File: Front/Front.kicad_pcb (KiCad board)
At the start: 2 copper layers, 75 x 75 mm, 0 parts

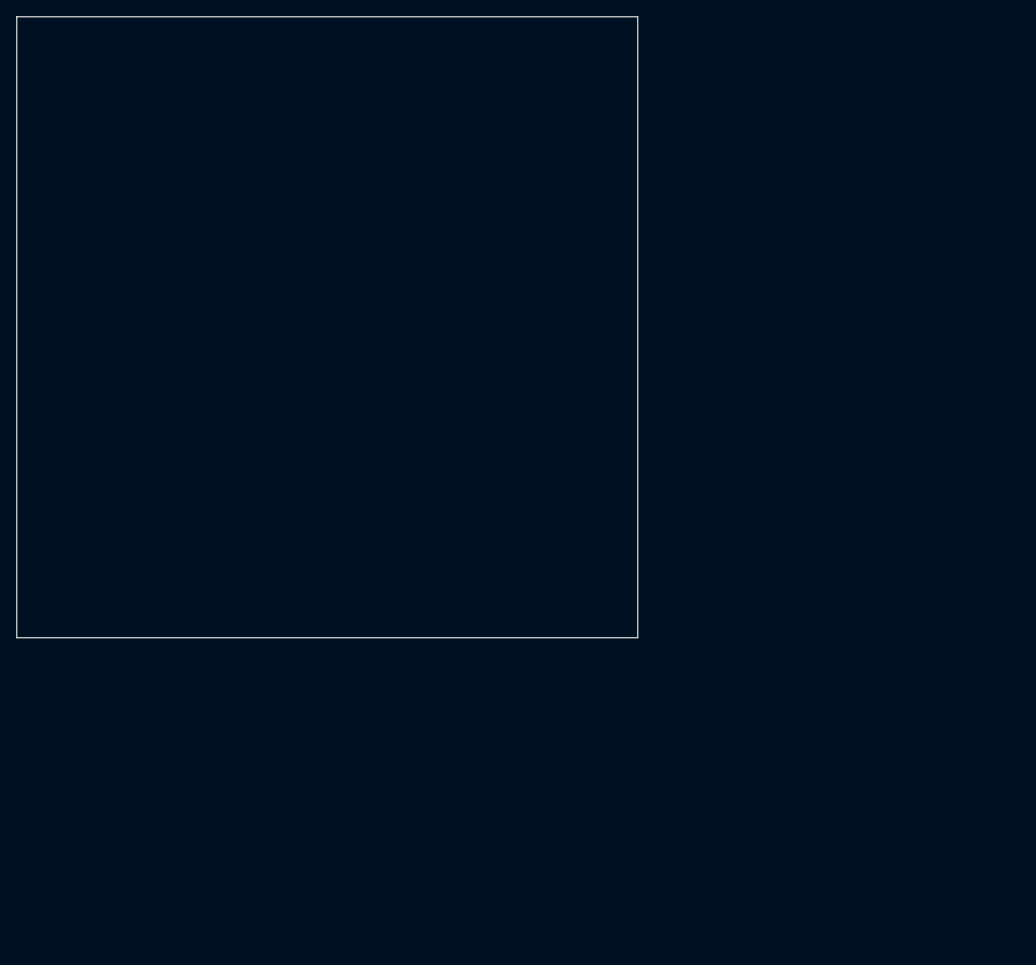
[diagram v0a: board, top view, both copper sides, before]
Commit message: a bunch of stuff
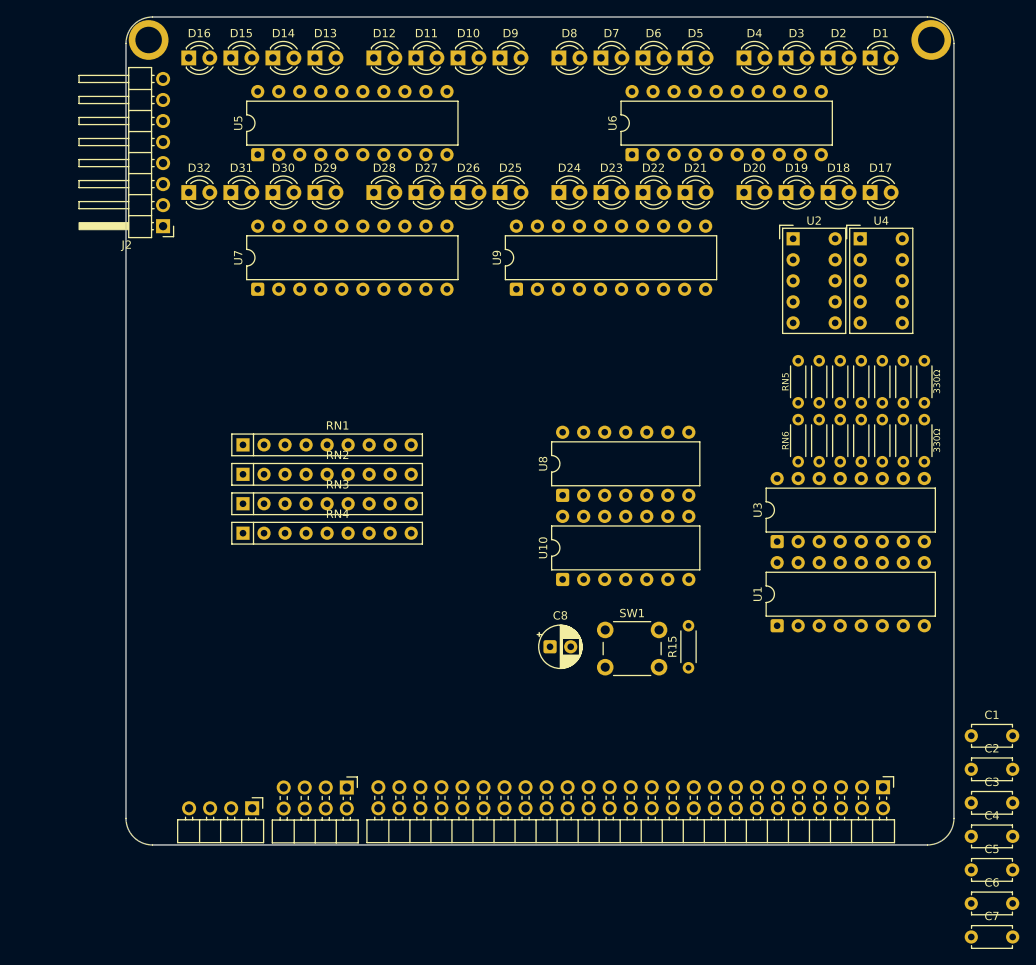
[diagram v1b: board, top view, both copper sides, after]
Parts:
- added C1: 100nF, Capacitor_THT:C_Disc_D4.7mm_W2.5mm_P5.00mm, F.Cu at (140.3, 111.8)
- added C2: 100nF, Capacitor_THT:C_Disc_D4.7mm_W2.5mm_P5.00mm, F.Cu at (140.3, 115.9)
- added C3: 100nF, Capacitor_THT:C_Disc_D4.7mm_W2.5mm_P5.00mm, F.Cu at (140.3, 119.9)
- added C4: 100nF, Capacitor_THT:C_Disc_D4.7mm_W2.5mm_P5.00mm, F.Cu at (140.3, 124.0)
- added C5: 100nF, Capacitor_THT:C_Disc_D4.7mm_W2.5mm_P5.00mm, F.Cu at (140.3, 128.0)
- added C6: 100nF, Capacitor_THT:C_Disc_D4.7mm_W2.5mm_P5.00mm, F.Cu at (140.3, 132.1)
- added C7: 100nF, Capacitor_THT:C_Disc_D4.7mm_W2.5mm_P5.00mm, F.Cu at (140.3, 136.1)
- added C8: 1µF, Capacitor_THT:CP_Radial_D5.0mm_P2.50mm, F.Cu at (89.4, 101.1)
- added D1: A0, LED_THT:LED_D3.0mm, F.Cu at (128.1, 30.0)
- added D10: A9, LED_THT:LED_D3.0mm, F.Cu at (78.3, 30.0)
- added D11: A10, LED_THT:LED_D3.0mm, F.Cu at (73.2, 30.0)
- added D12: A11, LED_THT:LED_D3.0mm, F.Cu at (68.1, 30.0)
- added D13: A12, LED_THT:LED_D3.0mm, F.Cu at (61.0, 30.0)
- added D14: A13, LED_THT:LED_D3.0mm, F.Cu at (55.9, 30.0)
- added D15: A14, LED_THT:LED_D3.0mm, F.Cu at (50.9, 30.0)
- added D16: A15, LED_THT:LED_D3.0mm, F.Cu at (45.8, 30.0)
- added D17: D0, LED_THT:LED_D3.0mm_Clear, F.Cu at (128.1, 46.2)
- added D18: D1, LED_THT:LED_D3.0mm_Clear, F.Cu at (123.0, 46.2)
- added D19: D2, LED_THT:LED_D3.0mm_Clear, F.Cu at (117.9, 46.2)
- added D2: A1, LED_THT:LED_D3.0mm, F.Cu at (123.0, 30.0)
- added D20: D3, LED_THT:LED_D3.0mm_Clear, F.Cu at (112.8, 46.2)
- added D21: D4, LED_THT:LED_D3.0mm_Clear, F.Cu at (105.7, 46.2)
- added D22: D5, LED_THT:LED_D3.0mm_Clear, F.Cu at (100.6, 46.2)
- added D23: D6, LED_THT:LED_D3.0mm_Clear, F.Cu at (95.6, 46.2)
- added D24: D7, LED_THT:LED_D3.0mm_Clear, F.Cu at (90.5, 46.2)
- added D25: RAM, LED_THT:LED_D3.0mm, F.Cu at (83.4, 46.2)
- added D26: ROM, LED_THT:LED_D3.0mm, F.Cu at (78.3, 46.2)
- added D27: BANK, LED_THT:LED_D3.0mm, F.Cu at (73.2, 46.2)
- added D28: IO, LED_THT:LED_D3.0mm, F.Cu at (68.1, 46.2)
- added D29: RESET, LED_THT:LED_D3.0mm, F.Cu at (61.0, 46.2)
- added D3: A2, LED_THT:LED_D3.0mm, F.Cu at (117.9, 30.0)
- added D30: NMI, LED_THT:LED_D3.0mm, F.Cu at (55.9, 46.2)
- added D31: HALT, LED_THT:LED_D3.0mm, F.Cu at (50.9, 46.2)
- added D32: WRITE, LED_THT:LED_D3.0mm, F.Cu at (45.8, 46.2)
- added D4: A3, LED_THT:LED_D3.0mm, F.Cu at (112.8, 30.0)
- added D5: A4, LED_THT:LED_D3.0mm, F.Cu at (105.7, 30.0)
- added D6: A5, LED_THT:LED_D3.0mm, F.Cu at (100.6, 30.0)
- added D7: A6, LED_THT:LED_D3.0mm, F.Cu at (95.6, 30.0)
- added D8: A7, LED_THT:LED_D3.0mm, F.Cu at (90.5, 30.0)
- added D9: A8, LED_THT:LED_D3.0mm, F.Cu at (83.4, 30.0)
- added J1: Buss, 0-Footprints:Card, F.Cu at (38.2, 25.0)
- added J2: Bank, Connector_PinHeader_2.54mm:PinHeader_1x08_P2.54mm_Horizontal, F.Cu at (42.7, 50.3)
- added R15: 10K, Resistor_THT:R_Axial_DIN0204_L3.6mm_D1.6mm_P5.08mm_Horizontal, F.Cu at (106.1, 103.6)
- added RN1: 330Ω, Resistor_THT:R_Array_SIP9, F.Cu at (52.3, 76.7)
- added RN2: 330Ω, Resistor_THT:R_Array_SIP9, F.Cu at (52.3, 80.3)
- added RN3: 330Ω, Resistor_THT:R_Array_SIP9, F.Cu at (52.3, 83.8)
- added RN4: 330Ω, Resistor_THT:R_Array_SIP9, F.Cu at (52.3, 87.4)
- added RN5: 330Ω, 0-Footprints:Resistor Pack 7, F.Cu at (119.4, 71.6)
- added RN6: 330Ω, 0-Footprints:Resistor Pack 7, F.Cu at (119.4, 78.7)
- added SW1: RESET, Button_Switch_THT:SW_PUSH_6mm, F.Cu at (96.1, 99.1)
- added U1: DM9368, Package_DIP:DIP-16_W7.62mm, F.Cu at (116.8, 98.6)
- added U10: 74HC14, Package_DIP:DIP-14_W7.62mm, F.Cu at (90.9, 93.0)
- added U2: Low Bank, Display_7Segment:HDSP-7401, F.Cu at (118.8, 51.8)
- added U3: DM9368, Package_DIP:DIP-16_W7.62mm, F.Cu at (116.8, 88.4)
- added U4: High Bank, Display_7Segment:HDSP-7401, F.Cu at (126.9, 51.8)
- added U5: 74LS240, Package_DIP:DIP-20_W7.62mm, F.Cu at (54.1, 41.7)
- added U6: 74LS240, Package_DIP:DIP-20_W7.62mm, F.Cu at (99.3, 41.7)
- added U7: 74LS240, Package_DIP:DIP-20_W7.62mm, F.Cu at (54.1, 57.9)
- added U8: 74LS00, Package_DIP:DIP-14_W7.62mm, F.Cu at (90.9, 82.8)
- added U9: 74LS245, Package_DIP:DIP-20_W7.62mm, F.Cu at (85.3, 57.9)
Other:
- board size 75 x 75 mm -> 100 x 100 mm
